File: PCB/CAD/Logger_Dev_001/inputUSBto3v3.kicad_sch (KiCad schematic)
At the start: 3 parts, among them J4 Connector, USB-TYPE-C-16P, U4 MCP2221AxSL, U6 XC6206P332MR

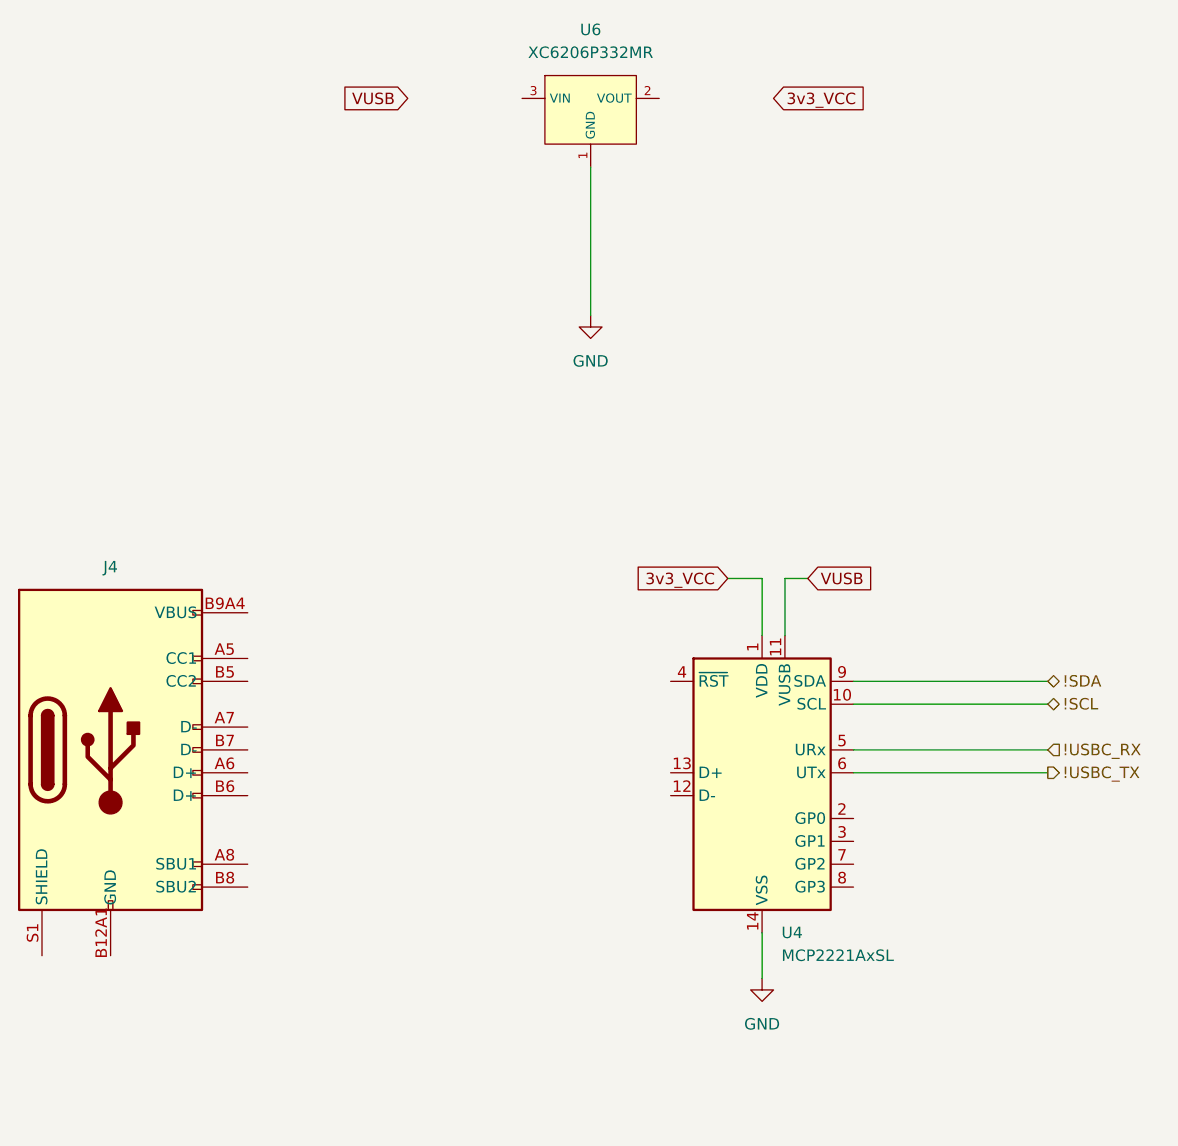
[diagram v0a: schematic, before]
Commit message: Library Submodule Update
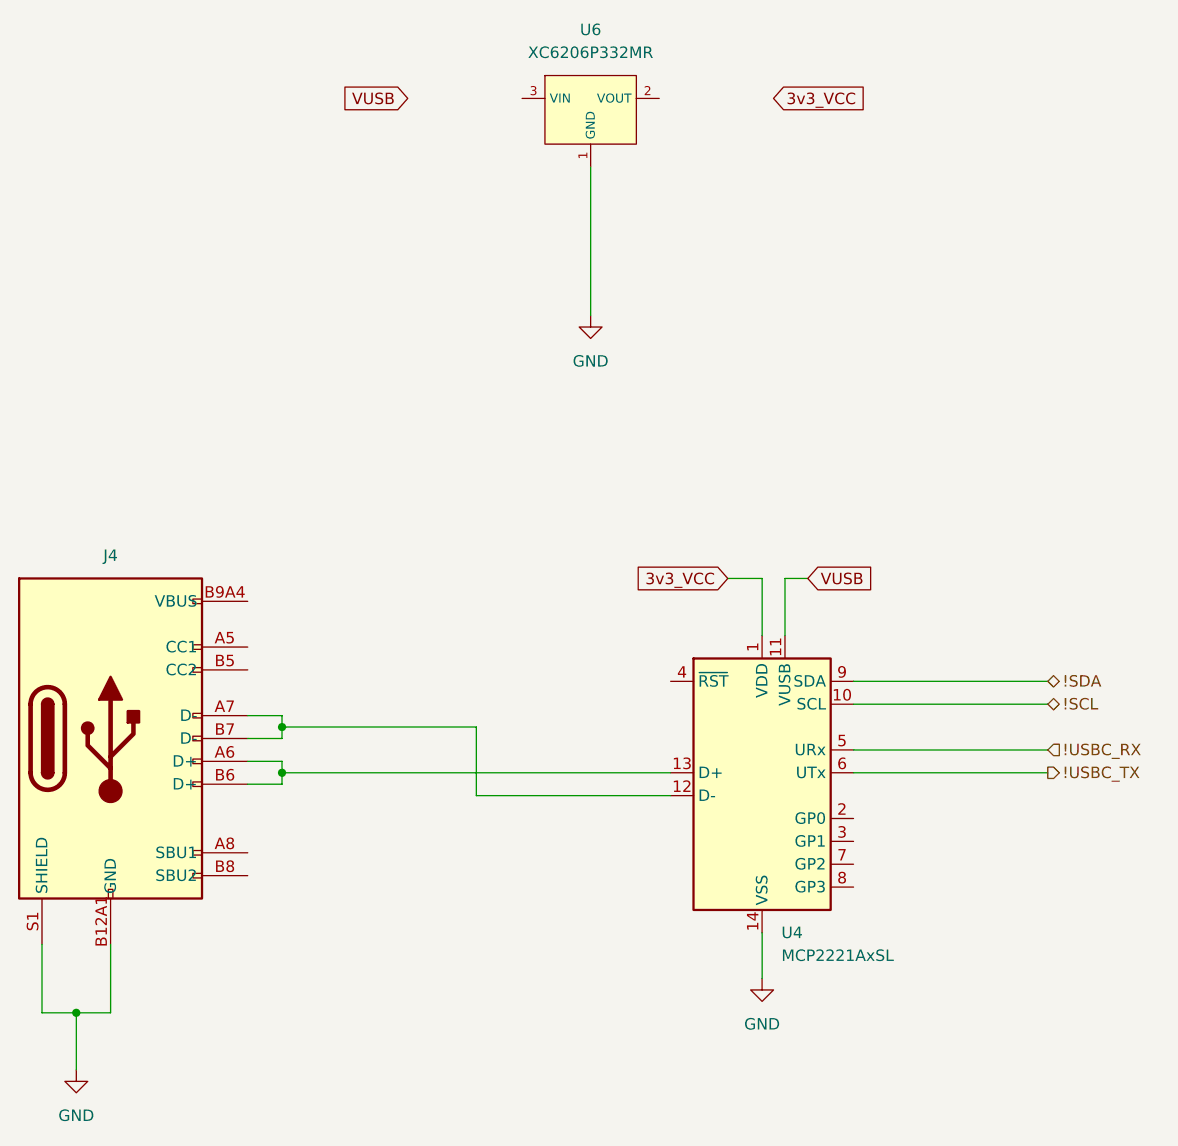
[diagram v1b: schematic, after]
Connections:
- net GND: now also J4.A12B1 (GND), J4.B12A1 (GND), J4.S1 (SHIELD)
- net at J4.A6 (D+): now also J4.B6 (D+), U4.13 (D+)
- net at J4.A7 (D-): now also J4.B7 (D-), U4.12 (D-)
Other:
- moved on the sheet: J4
